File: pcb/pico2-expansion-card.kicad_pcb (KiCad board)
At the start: 2 copper layers, 26 x 30.9 mm, 50 parts, among them J3 Conn_01x03_Socket, J4 Conn_01x04_Socket, Q1 EM6K6, Q2 EM6K6, SW1 SW_Push, U2 RP2354A, U4 AP2127K-3.3, Y1 ABM8-272-T3

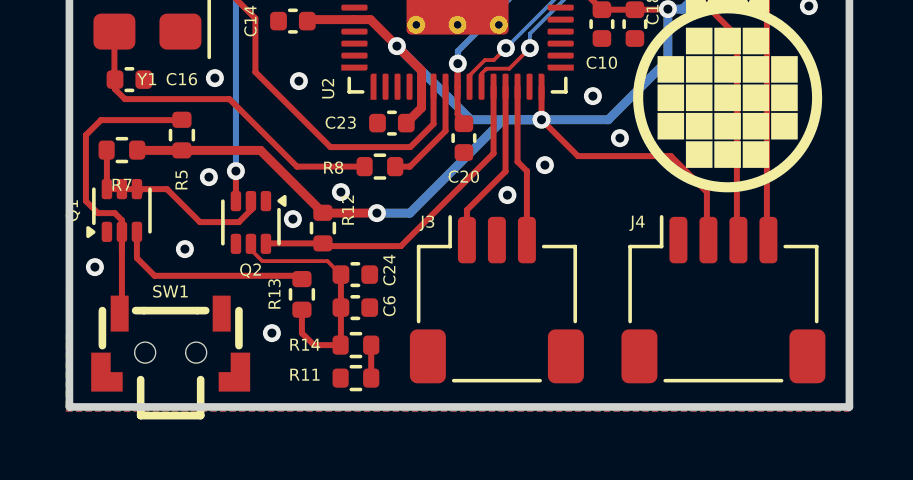
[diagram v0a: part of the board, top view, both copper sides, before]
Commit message: gerber and centroid
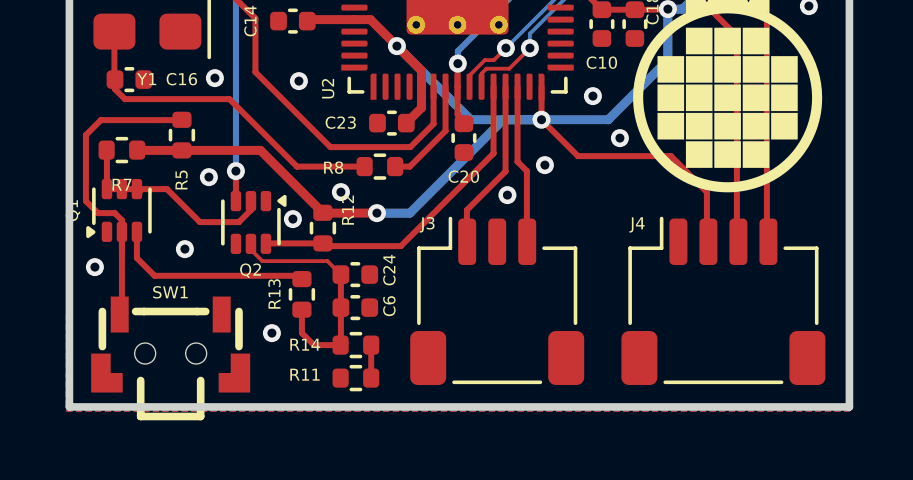
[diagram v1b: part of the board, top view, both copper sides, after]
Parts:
- moved J3 0.06 mm to (151.0, 144.5)
- moved J4 0.06 mm to (158.6, 144.5)
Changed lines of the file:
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@@
 	(footprint "Connector_JST:JST_SH_SM03B-SRSS-TB_1x03-1MP_P1.00mm_Horizontal"
 		(layer "F.Cu")
-		(at 151.02 144.45)
+		(at 151.03 144.505)
 		(descr "JST SH series connector, SM03B-SRSS-TB (http://www.jst-mfg.com/product/pdf/eng/eSH.pdf)")
 		(tags "connector JST SH horizontal")
@@
 	(footprint "pico2parts:BUTTON-SW-SMD_2P-TS24CA"
 		(layer "F.Cu")
-		(at 140.145 145.875 180)
+		(at 140.145 145.905 180)
 		(property "Reference" "SW1"
 			(at 0.00005 1.7 0)
@@
 			(polygon
 				(pts
-					(xy 140.5516 144.8512) (xy 140.5506 145.0511) (xy 139.7504 145.0502) (xy 139.7497 144.8505) (xy 138.6497 144.8505)
-					(xy 138.6497 144.7505) (xy 138.2508 144.7503) (xy 138.2505 144.8501) (xy 137.8707 144.8476) (xy 137.8703 147.1494)
-					(xy 138.2484 147.1519) (xy 138.2691 147.3511) (xy 138.5301 147.3501) (xy 138.5505 147.15) (xy 139.0182 147.1525)
-					(xy 139.0067 148.427) (xy 141.2689 148.4272) (xy 141.2732 147.2288) (xy 142.4249 147.2263) (xy 142.4201 144.8498)
-					(xy 142.0499 144.8502) (xy 142.049 144.751) (xy 141.651 144.7509) (xy 141.6507 144.8502) (xy 140.551 144.851)
+					(xy 140.5516 144.8812) (xy 140.5506 145.0811) (xy 139.7504 145.0802) (xy 139.7497 144.8805) (xy 138.6497 144.8805)
+					(xy 138.6497 144.7805) (xy 138.2508 144.7803) (xy 138.2505 144.8801) (xy 137.8707 144.8776) (xy 137.8703 147.1794)
+					(xy 138.2484 147.1819) (xy 138.2691 147.3811) (xy 138.5301 147.3801) (xy 138.5505 147.18) (xy 139.0182 147.1825)
+					(xy 139.0067 148.457) (xy 141.2689 148.4572) (xy 141.2732 147.2588) (xy 142.4249 147.2563) (xy 142.4201 144.8798)
+					(xy 142.0499 144.8802) (xy 142.049 144.781) (xy 141.651 144.7809) (xy 141.6507 144.8802) (xy 140.551 144.881)
 				)
 			)
@@
 			(polygon
 				(pts
-					(xy 138.2702 144.75) (xy 138.6202 144.75) (xy 138.6202 145.5) (xy 138.2702 145.5)
+					(xy 138.2702 144.78) (xy 138.6202 144.78) (xy 138.6202 145.53) (xy 138.2702 145.53)
 				)
 			)
@@
 			(polygon
 				(pts
-					(xy 141.6702 144.75) (xy 142.0202 144.75) (xy 142.0202 145.5) (xy 141.6702 145.5)
+					(xy 141.6702 144.78) (xy 142.0202 144.78) (xy 142.0202 145.53) (xy 141.6702 145.53)
 				)
 			)
@@
 			(polygon
 				(pts
-					(xy 137.87 146.15) (xy 137.87 147.15) (xy 138.5451 147.15) (xy 138.5451 147.04) (xy 137.9801 147.04)
-					(xy 137.9801 146.15)
+					(xy 137.87 146.18) (xy 137.87 147.18) (xy 138.5451 147.18) (xy 138.5451 147.07) (xy 137.9801 147.07)
+					(xy 137.9801 146.18)
 				)
 			)
@@
 			(polygon
 				(pts
-					(xy 142.4204 146.15) (xy 142.4204 147.15) (xy 141.7454 147.15) (xy 141.7454 147.04) (xy 142.3103 147.04)
-					(xy 142.3103 146.15)
+					(xy 142.4204 146.18) (xy 142.4204 147.18) (xy 141.7454 147.18) (xy 141.7454 147.07) (xy 142.3103 147.07)
+					(xy 142.3103 146.18)
 				)
 			)
@@
 	(footprint "Connector_JST:JST_SH_SM04B-SRSS-TB_1x04-1MP_P1.00mm_Horizontal"
 		(layer "F.Cu")
-		(at 158.57 144.45)
+		(at 158.57 144.505)
 		(descr "JST SH series connector, SM04B-SRSS-TB (http://www.jst-mfg.com/product/pdf/eng/eSH.pdf)")
 		(tags "connector JST SH horizontal")
